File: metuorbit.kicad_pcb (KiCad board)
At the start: 2 copper layers, 120 x 120 mm, 24 parts, among them IC1 BLACKPILLF4, IC2 LoRa E220-900T30D, IC3 BNO055, IC4 NEO-M8N, IC5 BMP388, IC6 MicroSD_Reader, IC7 HT7333, IC8 MP1584, J1 Resistive Wire, J2 BATT Input, J3 SERVO1, J4 SERVO2, Q1 2N3904, Q2 IRLZ44N

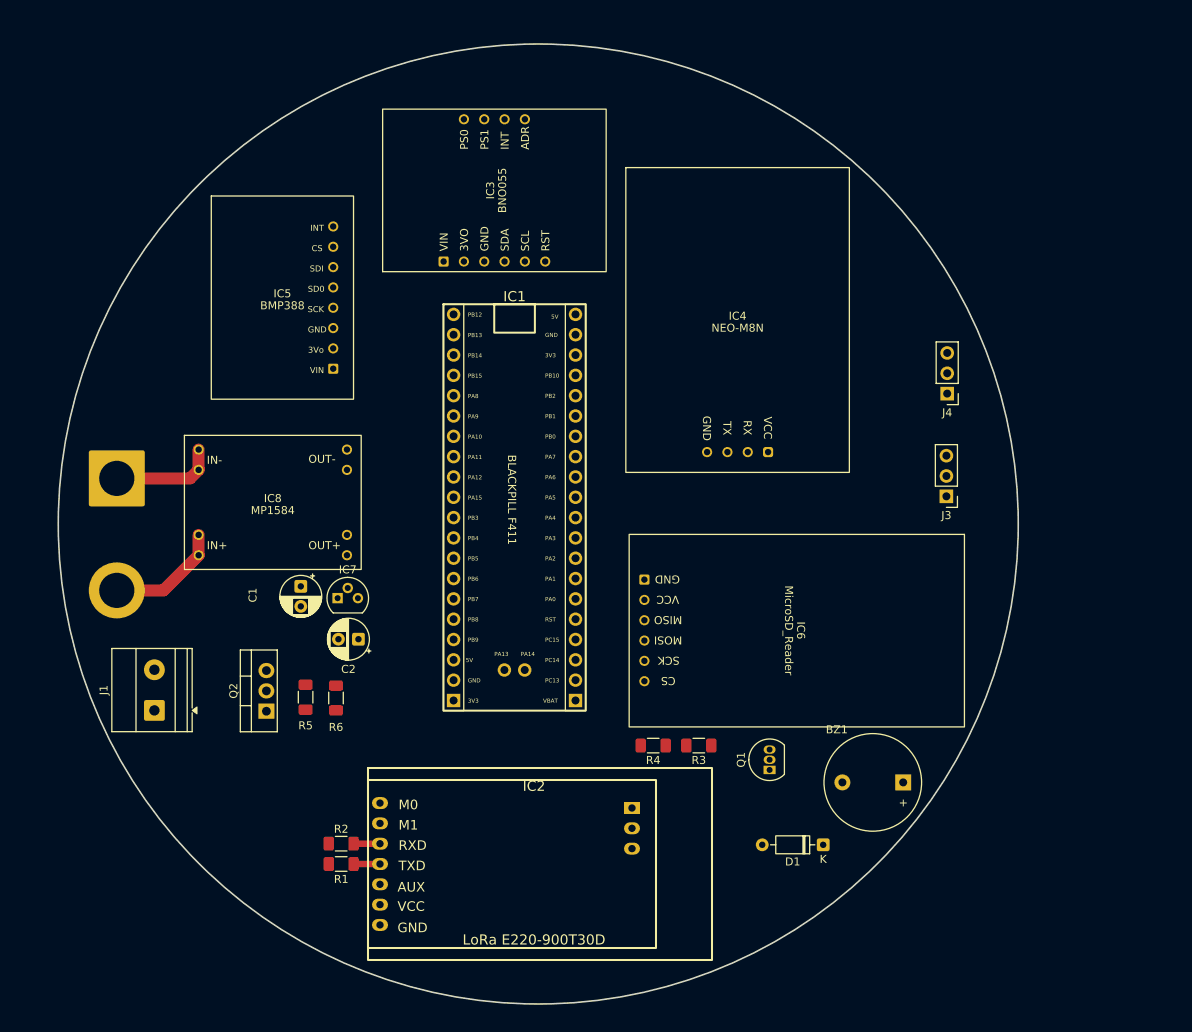
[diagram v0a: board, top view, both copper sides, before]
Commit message: First design of PCB is done.
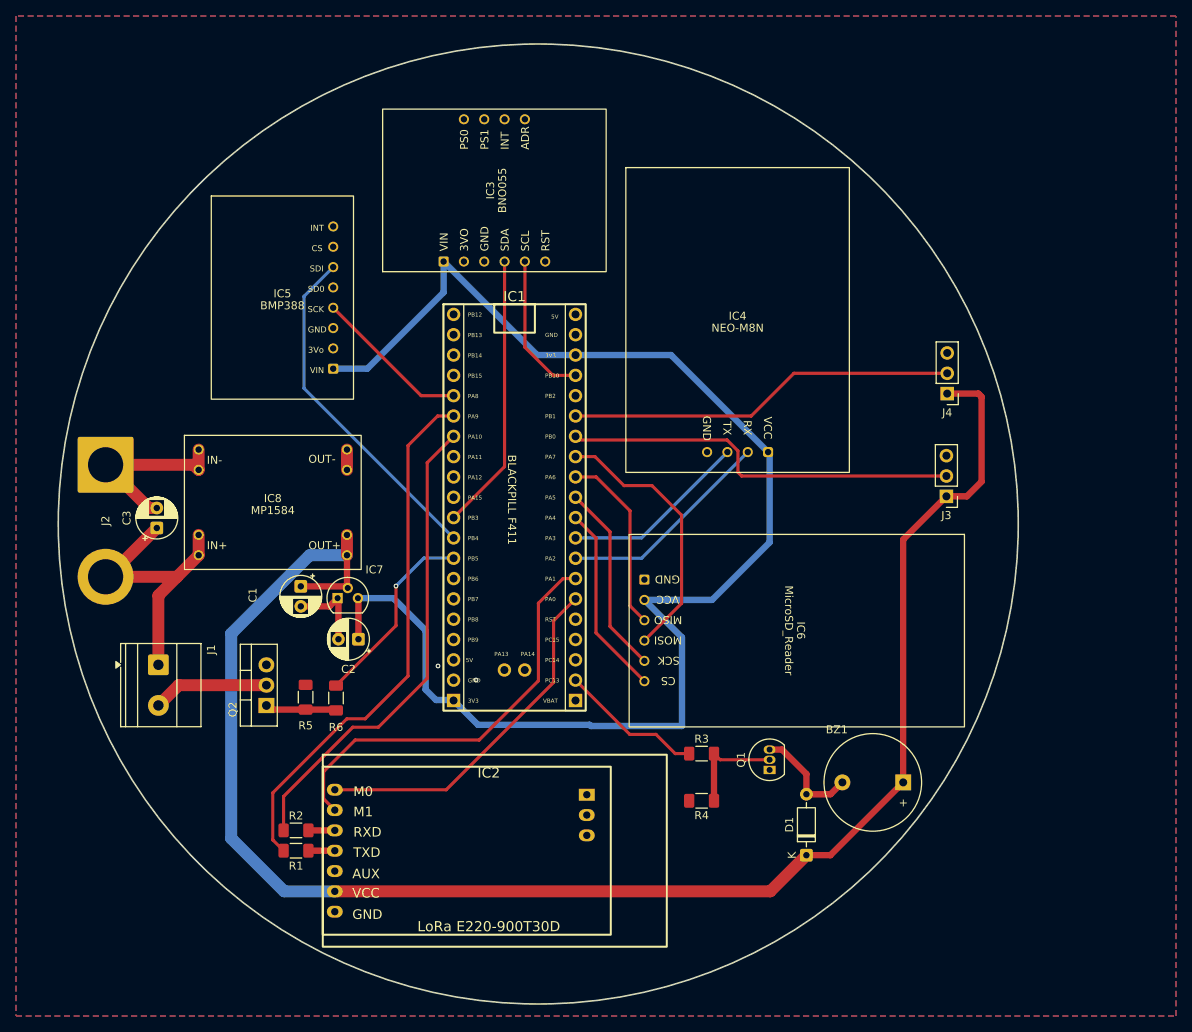
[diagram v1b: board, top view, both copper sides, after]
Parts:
- added C3: 470u, Capacitor_THT:CP_Radial_D5.0mm_P2.50mm, F.Cu at (157.6, 159.0)
- J2: moved to F.Cu
- moved R4 9.18 mm to (225.7, 193.1)
- moved IC2 5.89 mm to (179.9, 191.7)
- moved R1 5.89 mm to (175.0, 199.3)
- moved R2 5.89 mm to (175.0, 196.8)
- moved J1 5.72 mm to (157.8, 176.1), turned to -90 degrees
- moved D1 2.47 mm to (238.8, 199.9), turned to 90 degrees
- moved J2 2.20 mm to (151.2, 151.1)
- moved R3 1.06 mm to (225.7, 187.2), turned to 0 degrees
- moved Q2 0.72 mm to (171.3, 181.2)
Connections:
- IC1 pad PA10: /LORA_TX -> /LORA_RX
- IC1 pad PA9: /LORA_RX -> /LORA_TX
- IC1 pad PB2: /TRIG -> unconnected-(IC1-PadPB2)
- IC1 pad PB5: unconnected-(IC1-PadPB5) -> /TRIG
- IC4 pad 1: GND -> +3V3
- IC4 pad 2: /NEO_TX -> /NEO_RX
- IC4 pad 3: /NEO_RX -> /NEO_TX
- IC4 pad 4: +3V3 -> GND
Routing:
- net +5V: track 0.00 -> 207.4 mm
- net +3V3: track 0.00 -> 176.4 mm
- net /LORA_TX: track 0.00 -> 66.8 mm
- net /LORA_RX: track 0.00 -> 59.9 mm
- net /LORA_M1: track 0.00 -> 52.6 mm
- net /SERVO1: track 0.00 -> 50.0 mm
- net /SERVO2: track 0.00 -> 48.7 mm
- net /LORA_M0: track 0.00 -> 44.5 mm
- net /BMP_SDA: track 0.00 -> 43.2 mm
- net /BNO_SDA: track 0.00 -> 34.6 mm
- net /SD_MOSI: track 0.00 -> 33.9 mm
- net /NEO_RX: track 0.00 -> 27.0 mm
- net /TRIG: track 0.00 -> 24.2 mm, vias 0 -> 1
- net /SD_SCK: track 0.00 -> 24.0 mm
- net /SD_CS: track 0.00 -> 24.0 mm
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- added copper zone on B.Cu, net GND
- added copper zone on F.Cu, net GND
